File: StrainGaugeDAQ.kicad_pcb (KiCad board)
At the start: 2 copper layers, 86.6 x 69.5 mm, 95 parts, among them J1 IN1, J2 IN2, J3 IN3, J4 IN4, J5 VBAT, J6 SPI+INT, U1 INA351CDSIDSGR, U2 MCP3562RT-E/NC, U3 INA351CDSIDSGR, U4 INA351CDSIDSGR, U5 INA351CDSIDSGR, U6 AP62150Z6, U7 AP2127K-3.3, U8 AP2127K-3.3

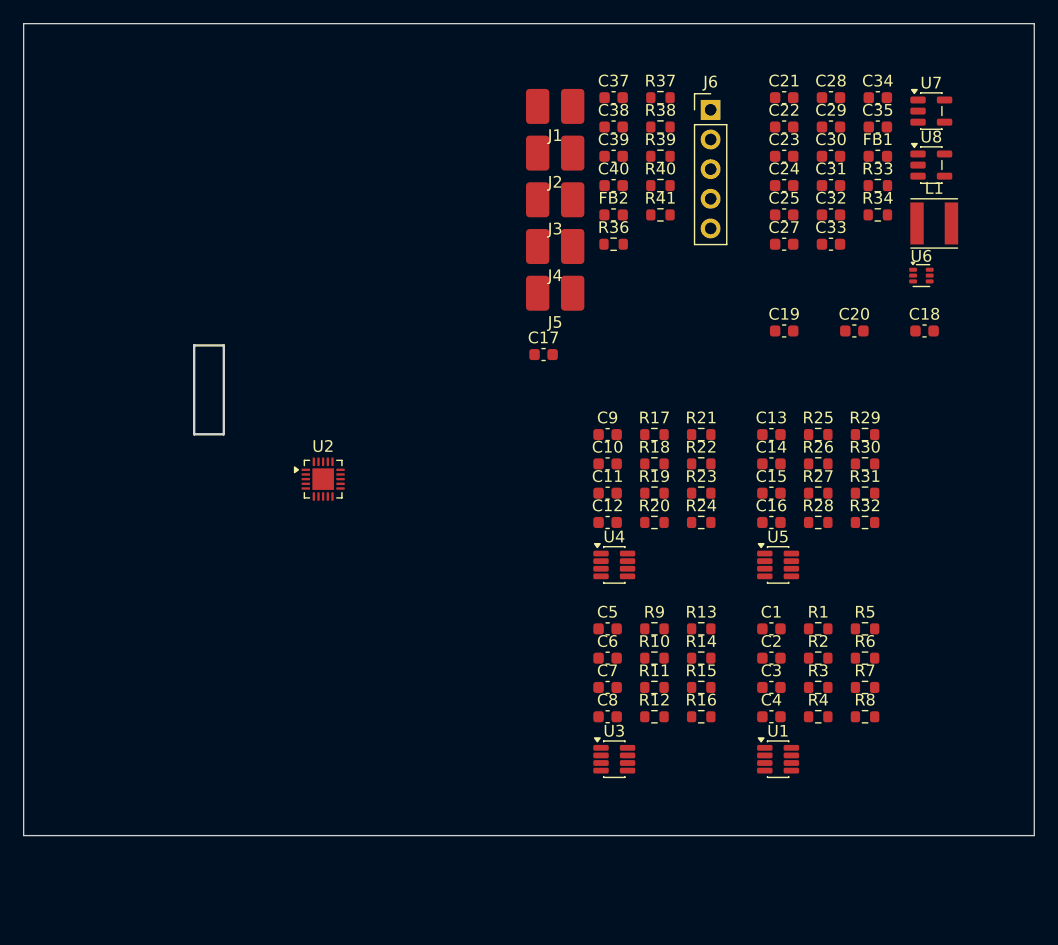
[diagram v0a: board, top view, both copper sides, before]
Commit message: Layout work
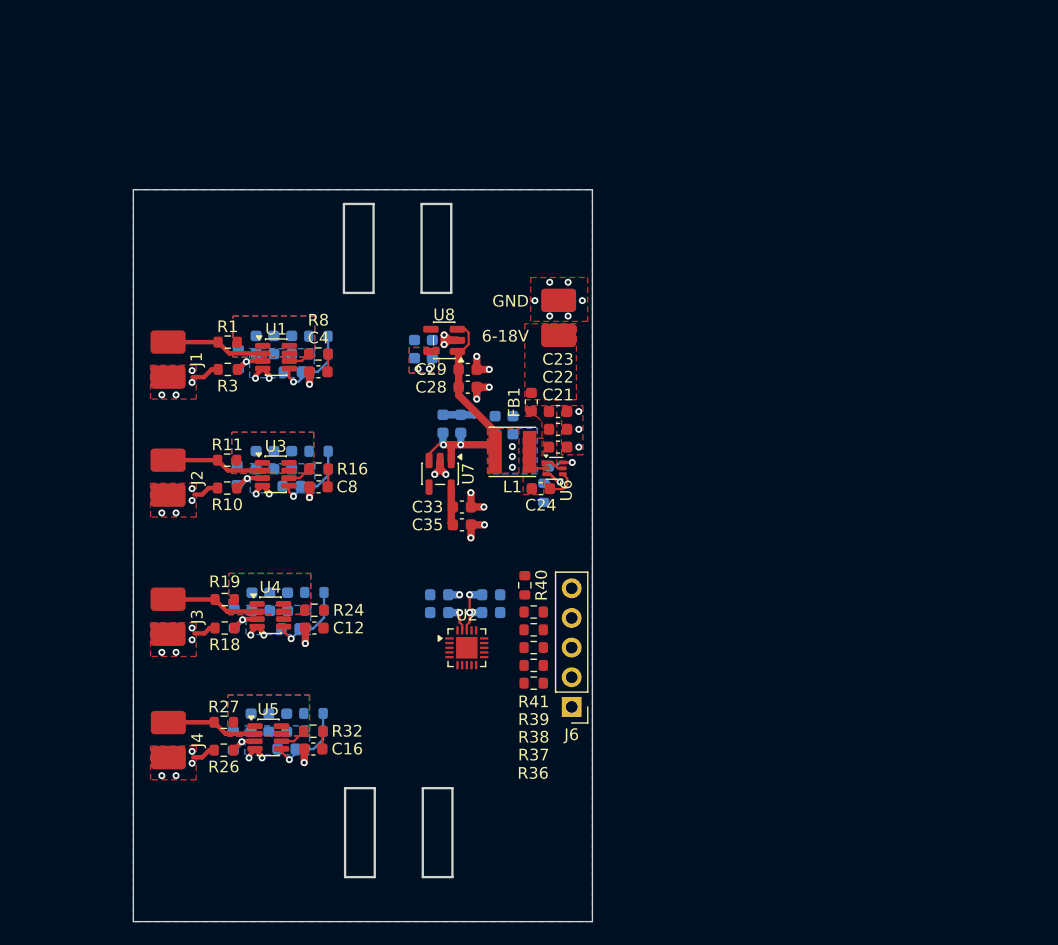
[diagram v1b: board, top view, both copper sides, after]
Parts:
- removed FB2: FerriteBead, Inductor_SMD:L_0603_1608Metric
- removed R12, R13, R20, R21, R28, R29, R6, R7: R_US, Resistor_SMD:R_0603_1608Metric
- C1, C10, C11, C13, C14, C15, C17, C18, C19, C2, C20, C3, C5, C6, C7, C9: value C -> 100n; moved to B.Cu
- C21, C22: value C -> 22u
- C23: value C -> 100n
- C25, C27, C30, C31, C32, C34, C37, C38, C39, C40, R17, R2, R25, R33, R34, R9: moved to B.Cu
- J5: value VBAT -> 6-18V
- R14, R15, R22, R23, R30, R31, R4, R5: value R_US -> 10k; moved to B.Cu
- moved C20 59.1 mm to (146.5, 112.6), turned to 90 degrees
- moved R3 57.4 mm to (141.4, 82.3), turned to 180 degrees
- moved R25 56.5 mm to (141.9, 114.1), turned to -90 degrees
- moved R26 56.5 mm to (141.1, 114.9), turned to 180 degrees
- moved R1 56.2 mm to (141.4, 80.0), turned to 180 degrees
- moved R8 56.2 mm to (149.2, 81.0), turned to 180 degrees
- moved R2 55.9 mm to (142.3, 81.4), turned to -90 degrees
- moved C18 55.3 mm to (146.9, 90.1), turned to 90 degrees
- moved U1 55.1 mm to (145.6, 81.2)
- moved R27 54.6 mm to (141.1, 112.5), turned to 180 degrees
- moved R4 53.8 mm to (149.2, 79.5)
- moved J4 53.7 mm to (136.3, 114.0), turned to 90 degrees
- moved J6 52.5 mm to (170.9, 111.2), turned to 180 degrees
- moved R5 52.4 mm to (149.2, 81.0), turned to 180 degrees
- moved U7 52.3 mm to (159.6, 91.2), turned to -90 degrees
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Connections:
- U1 pad 1: Net-(U1-GS) -> unconnected-(U1-GS-Pad1)
- U2 pad 1: Net-(U2-AGND) -> GND
- U2 pad 20: Net-(U2-AGND) -> GND
- U3 pad 1: Net-(U3-GS) -> unconnected-(U3-GS-Pad1)
- U4 pad 1: Net-(U4-GS) -> unconnected-(U4-GS-Pad1)
- U5 pad 1: Net-(U5-GS) -> unconnected-(U5-GS-Pad1)
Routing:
- net GND: track 0.00 -> 40.2 mm, vias 0 -> 50
- net 5V: track 0.00 -> 23.4 mm, vias 0 -> 5
- net DVDD: track 0.00 -> 8.57 mm, vias 0 -> 2
- net /Amp1/In+: track 0.00 -> 8.51 mm
- net /Amp2/In+: track 0.00 -> 8.45 mm
- net /Amp3/In+: track 0.00 -> 8.06 mm
- net /Amp4/In+: track 0.00 -> 7.83 mm
- net Net-(U1-REF): track 0.00 -> 7.46 mm, vias 0 -> 1
- net Net-(U5-REF): track 0.00 -> 7.26 mm, vias 0 -> 1
- net Net-(U4-REF): track 0.00 -> 7.10 mm, vias 0 -> 1
- net Net-(U3-REF): track 0.00 -> 6.99 mm, vias 0 -> 1
- net Net-(U1-IN+): track 0.00 -> 4.48 mm, vias 0 -> 1
- net Net-(U3-IN+): track 0.00 -> 3.62 mm, vias 0 -> 1
- net AVDD: track 0.00 -> 3.55 mm, vias 0 -> 4
- net Net-(U4-IN+): track 0.00 -> 3.28 mm, vias 0 -> 1
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- added copper zone on F.Cu, net /PD/VCC
- added copper zone on B.Cu, net 5V
- added copper zone on F.Cu, net 5V
- added copper zone on B.Cu, net AVDD
- added copper zone on F.Cu, net AVDD
- added copper zone on B.Cu, net GND
- added copper zone on F.Cu, net GND
- added copper zone on F.Cu, net Net-(U6-EN)
- added copper zone on F.Cu, net Net-(U6-SW)
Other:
- board size 86.6 x 69.5 mm -> 39.3 x 62.7 mm
- board text added: "CS"
- board text added: "GND"
- board text added: "IRQ"
- board text added: "SCLK"
- board text added: "SDI"
- board text added: "SDO"

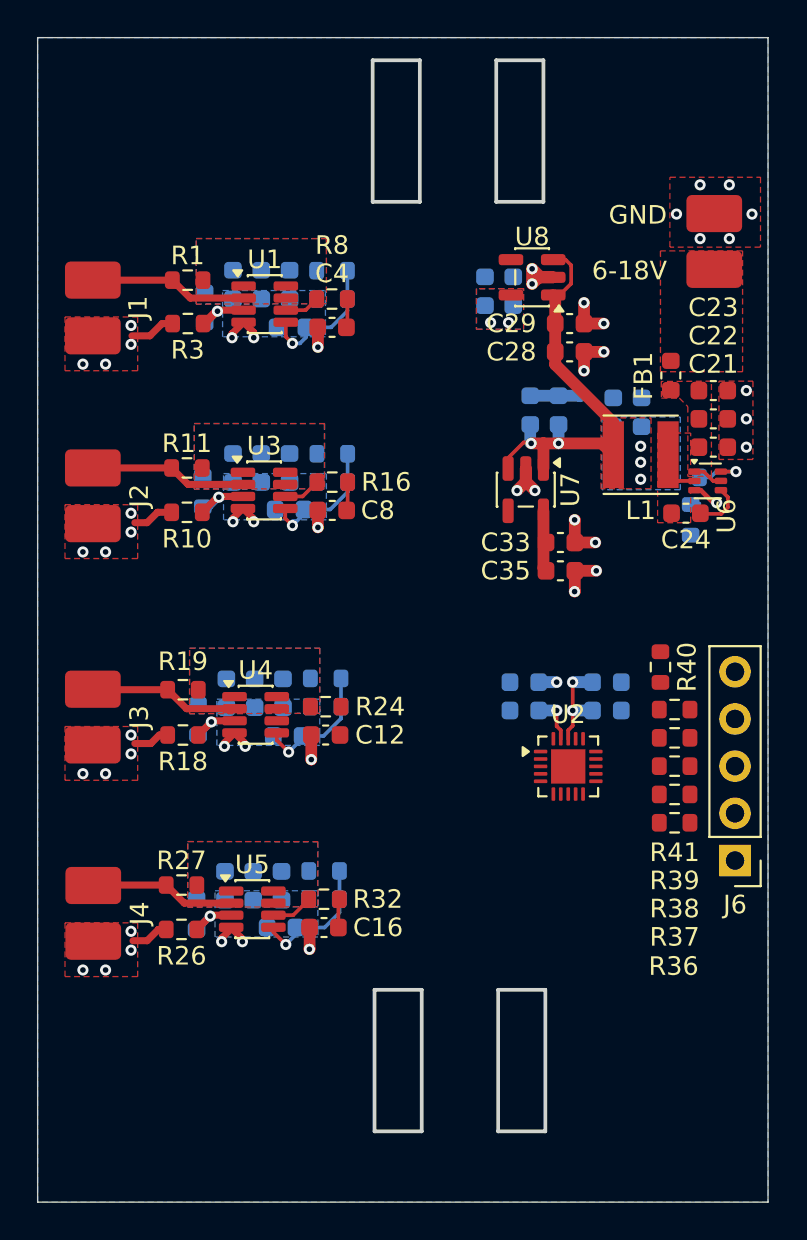
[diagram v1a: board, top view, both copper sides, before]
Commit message: fab files created
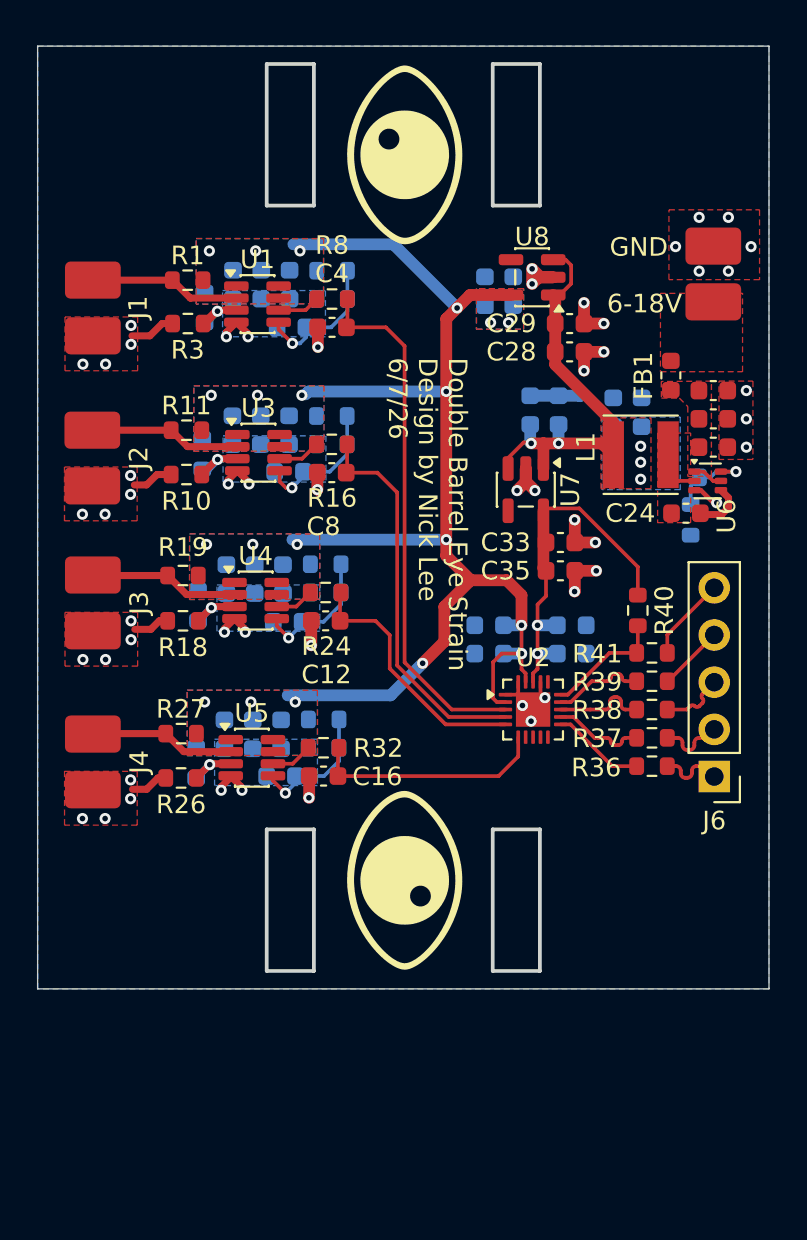
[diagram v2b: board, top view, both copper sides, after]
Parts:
- added H1: MountingScrew, AA-Custom:EyePicture, F.Cu at (153.1, 73.2)
- added H2: MountingScrew, AA-Custom:EyePicture, F.Cu at (153.1, 112.3)
- moved C15 8.15 mm to (146.5, 106.7)
- moved C16 8.15 mm to (148.7, 106.7)
- moved J4 8.15 mm to (136.3, 105.9)
- moved U5 8.15 mm to (144.9, 105.7)
- moved C13 8.15 mm to (143.4, 104.4)
- moved C14 8.15 mm to (144.9, 104.4)
- moved C20 8.15 mm to (146.5, 104.4)
- moved R25 8.15 mm to (141.9, 105.9)
- moved R26 8.15 mm to (141.1, 106.8)
- moved R27 8.15 mm to (141.1, 104.4)
- moved R30 8.15 mm to (148.8, 103.6)
- moved R31 8.15 mm to (148.7, 105.1)
- moved R32 8.15 mm to (148.7, 105.1)
- moved C10 6.15 mm to (145.0, 96.0)
- moved C11 6.15 mm to (146.8, 98.3)
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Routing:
- net AVDD: track 3.55 -> 72.5 mm, vias 4 -> 20
- net /Amp1/Vout: track 1.54 -> 28.6 mm
- net /Amp2/Vout: track 1.55 -> 21.0 mm
- net /Amp3/Vout: track 0.00 -> 13.8 mm
- net /Amp4/Vout: track 1.55 -> 12.7 mm
- net DVDD: track 8.57 -> 19.7 mm
- net Net-(U2-*IRQ/MDAT): track 0.00 -> 6.51 mm
- net Net-(U2-*CS): track 0.00 -> 5.02 mm
- net Net-(U2-SCK): track 0.00 -> 4.97 mm
- net Net-(U2-SDO): track 0.00 -> 4.97 mm
- net Net-(U2-SDI): track 0.00 -> 4.97 mm
- net Net-(J6-Pin_5): track 0.00 -> 4.55 mm
- net Net-(J6-Pin_4): track 0.00 -> 3.56 mm
- net Net-(J6-Pin_1): track 0.00 -> 3.56 mm
- net Net-(J6-Pin_2): track 0.00 -> 3.54 mm
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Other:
- board size 39.3 x 62.7 mm -> 39.4 x 50.7 mm
- board text added: "Double Barrel Eye Strain Design by Nick Lee 6/7/26"
